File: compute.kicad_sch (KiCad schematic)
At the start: 36 parts, among them J4 Micro_SD_Card_Det2, J7 Conn_01x03_Pin, SW1 BOOTSEL, SW2 USER, U1 RP2350_80QFN, U2 W25Q32JVZP, Y1 ABM8-272-T3

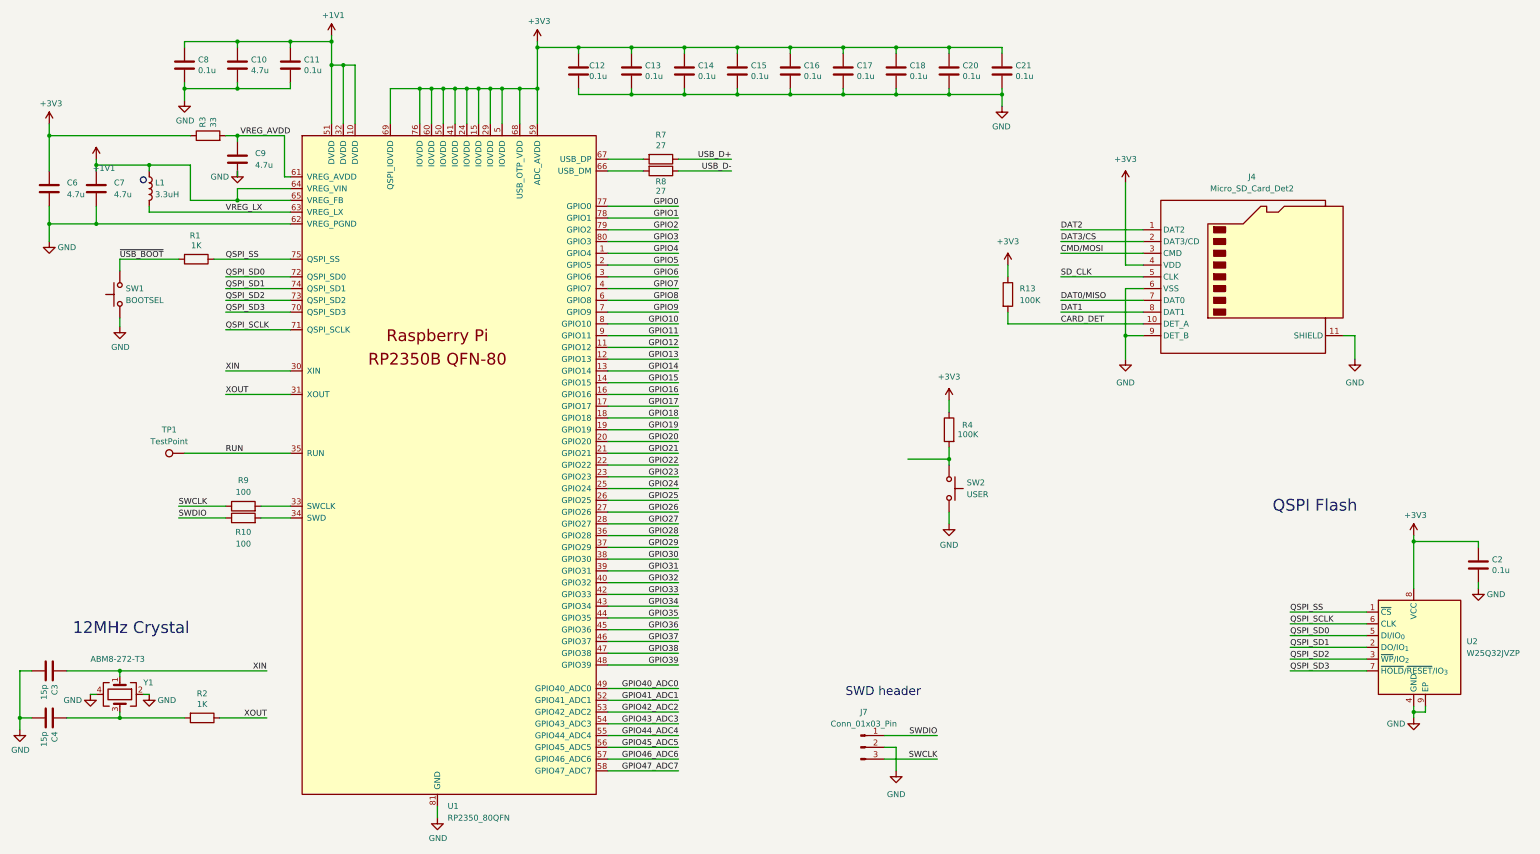
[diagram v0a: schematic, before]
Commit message: progress, particularly on power
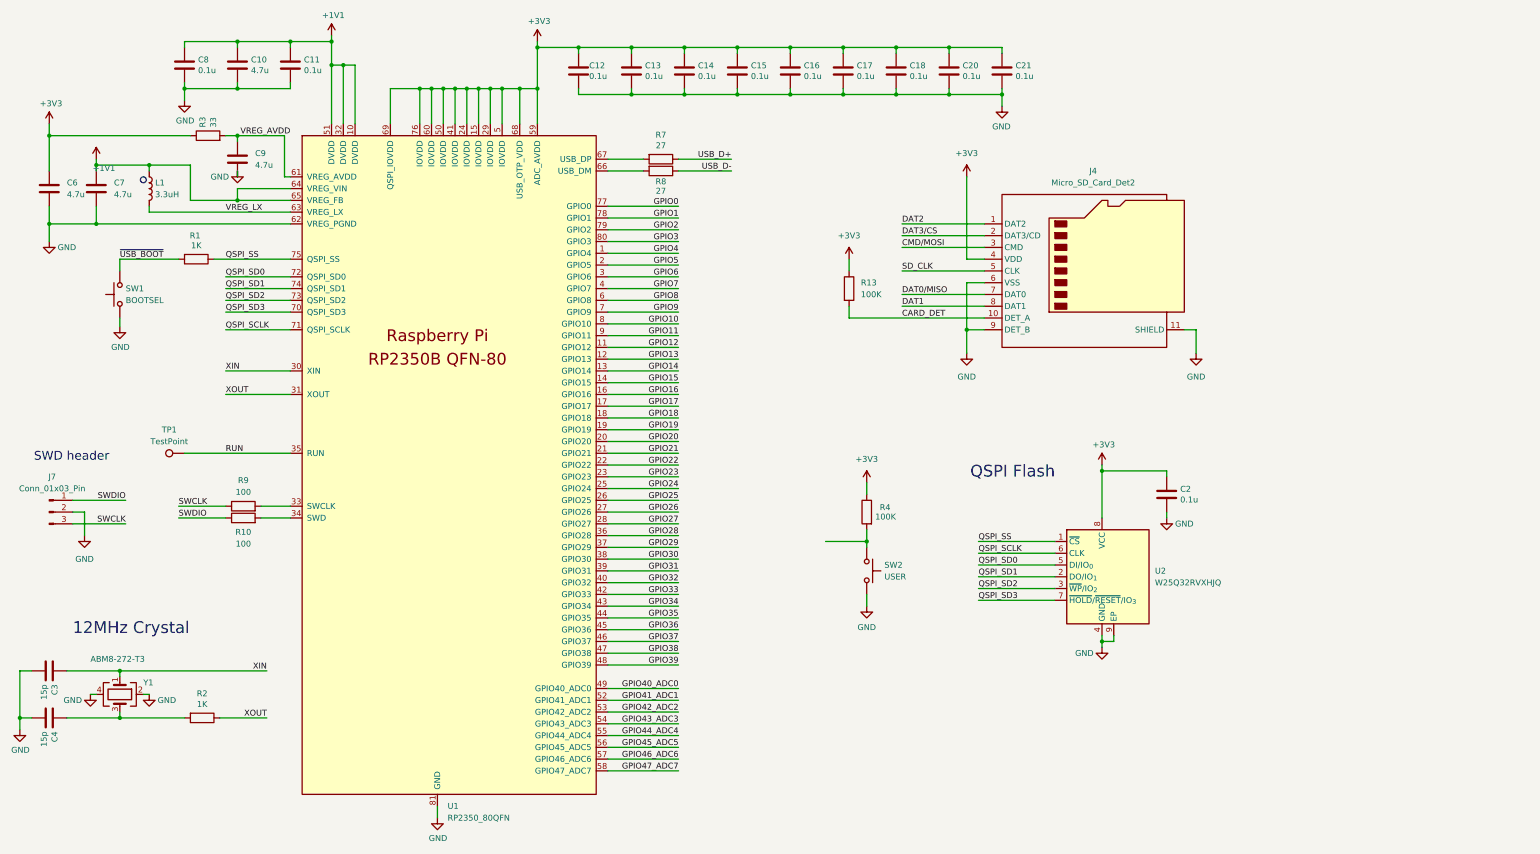
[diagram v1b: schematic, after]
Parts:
- U2: value W25Q32JVZP -> W25Q32RVXHJQ; footprint Package_SON:WSON-8-1EP_6x5mm_P1.27mm_EP3.4x4.3mm -> Package_SON:Winbond_USON-8-1EP_3x2mm_P0.5mm_EP0.2x1.6mm
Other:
- moved on the sheet: C2, J4, J7, R13, R4, SW2, U2
